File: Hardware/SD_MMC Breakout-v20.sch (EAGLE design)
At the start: 8 parts, among them U1 SD_CARD_SOCKET4UCON

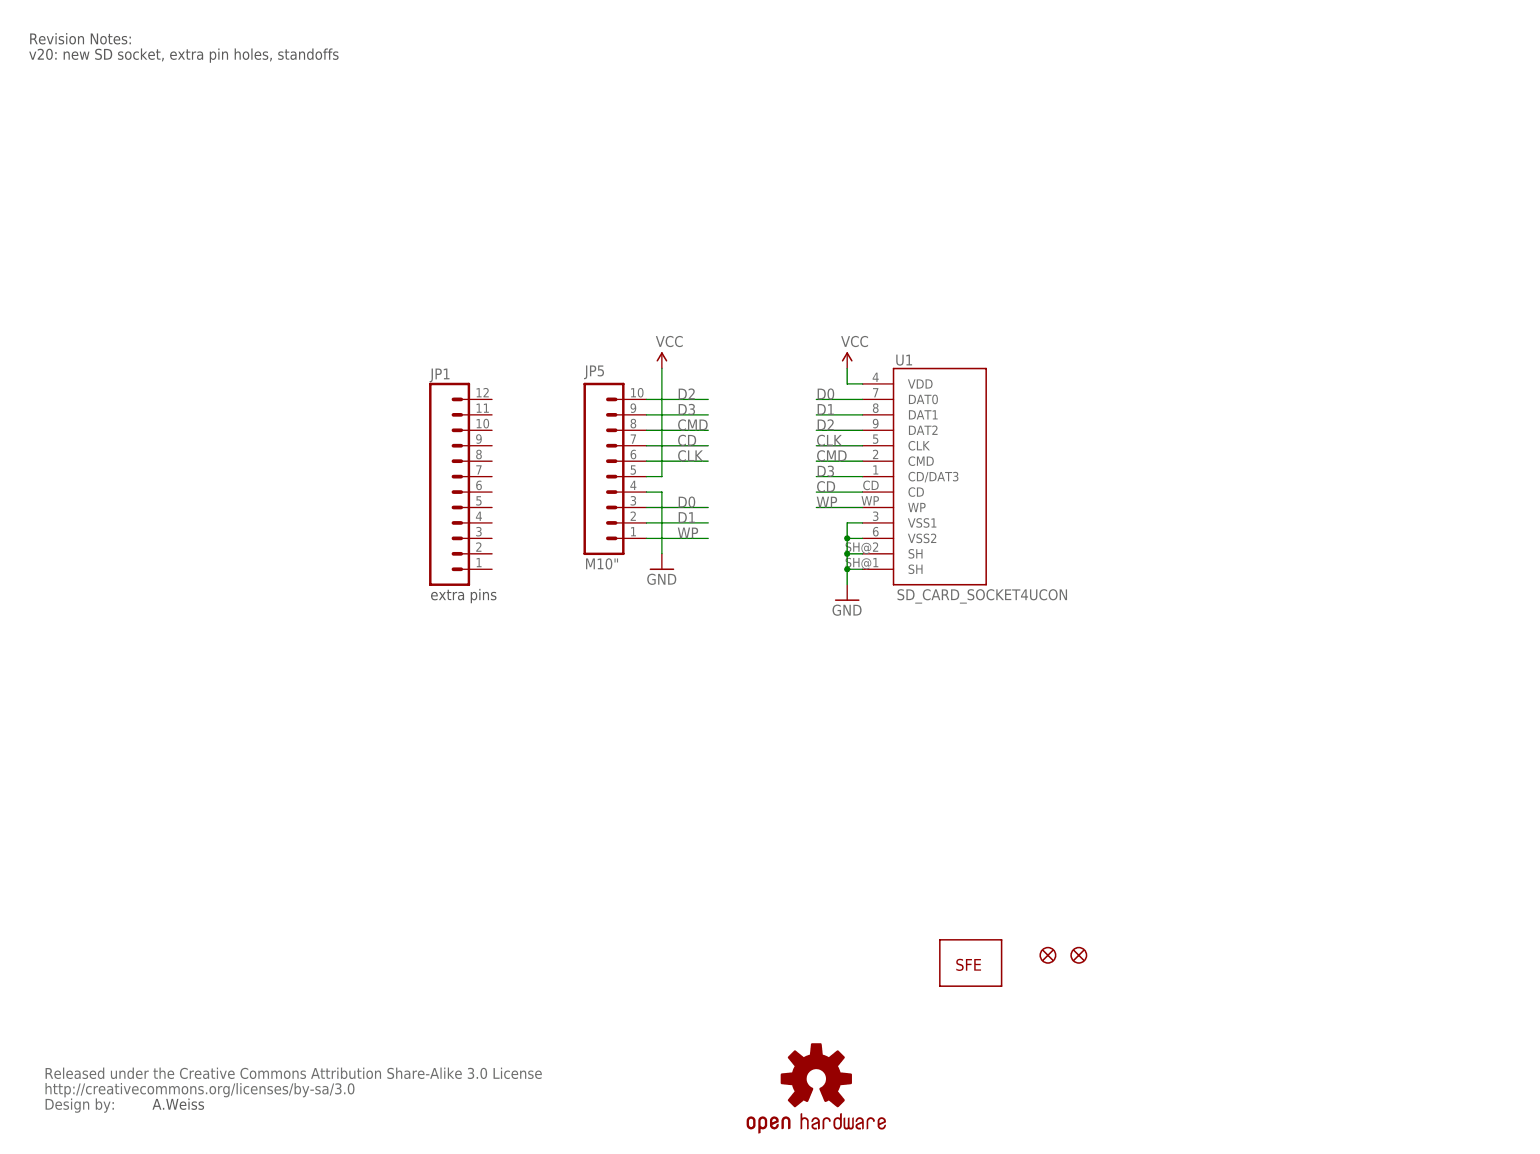
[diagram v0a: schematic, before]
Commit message: Added standoffs, sch work
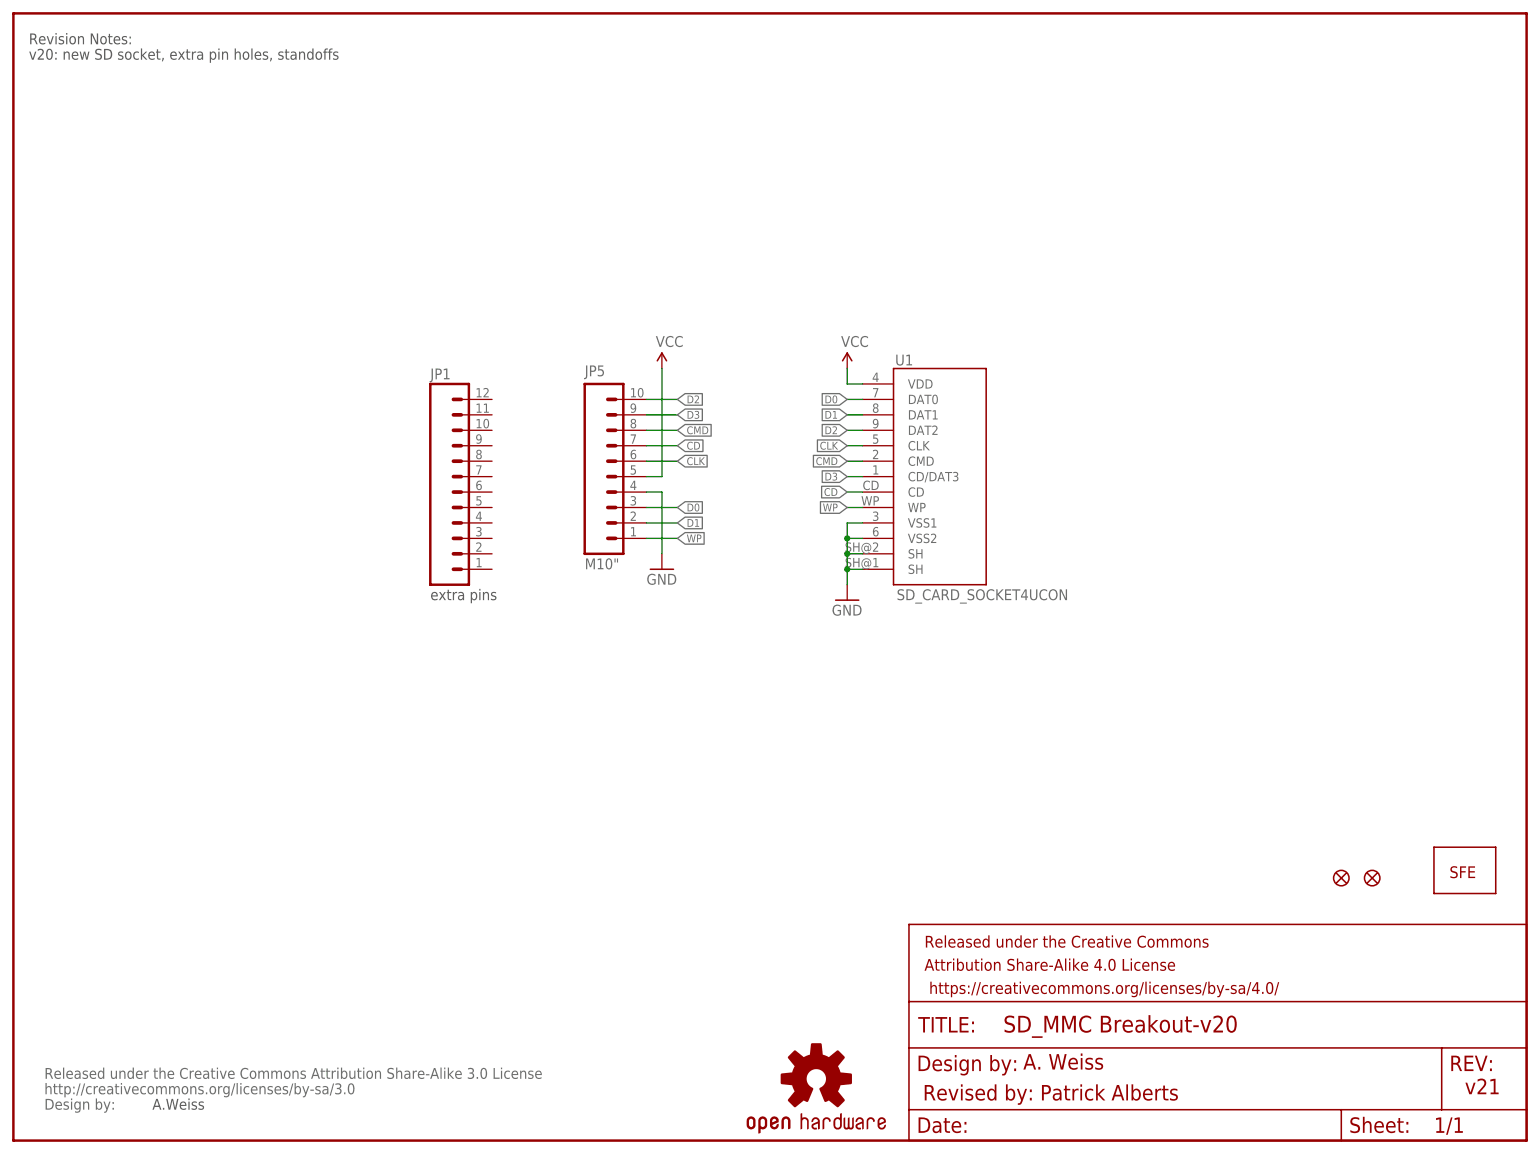
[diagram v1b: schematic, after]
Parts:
- added FRAME1: FRAME-LETTER, SparkFun-Aesthetics:FRAME-LETTER
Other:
- note added: "A. Weiss"
- note added: "Revised by: Patrick Alberts"
- note added: "v21"
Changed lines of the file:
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@@
 <?xml version="1.0" encoding="utf-8"?>
 <!DOCTYPE eagle SYSTEM "eagle.dtd">
-<eagle version="6.4">
+<eagle version="6.5.0">
 <drawing>
 <settings>
@@
 <layer number="106" name="bPlate" color="7" fill="1" visible="no" active="yes"/>
 <layer number="107" name="Crop" color="7" fill="1" visible="no" active="yes"/>
+<layer number="108" name="tplace-old" color="10" fill="1" visible="no" active="yes"/>
+<layer number="109" name="ref-old" color="11" fill="1" visible="no" active="yes"/>
 <layer number="116" name="Patch_BOT" color="9" fill="4" visible="yes" active="yes"/>
 <layer number="121" name="_tsilk" color="7" fill="1" visible="yes" active="yes"/>
@@
 <layer number="144" name="Drill_legend" color="7" fill="1" visible="no" active="yes"/>
 <layer number="151" name="HeatSink" color="7" fill="1" visible="yes" active="yes"/>
+<layer number="199" name="Contour" color="7" fill="1" visible="yes" active="yes"/>
 <layer number="200" name="200bmp" color="1" fill="10" visible="no" active="no"/>
 <layer number="201" name="201bmp" color="2" fill="1" visible="no" active="no"/>
@@
 </classes>
 <parts>
-<part name="FRAME1" library="SparkFun" deviceset="FRAME-LETTER" device=""/>
+<part name="FRAME1" library="SparkFun-Aesthetics" deviceset="FRAME-LETTER" device=""/>
 <part name="U$1" library="SparkFun" deviceset="LOGO-SFE" device="NEW"/>
 <part name="U1" library="SparkFun-Connectors" deviceset="SD_CARD_SOCKET" device="4UCON"/>
@@
 <text x="2.54" y="177.8" size="1.778" layer="97">v20: new SD socket, extra pin holes, standoffs</text>
 <text x="68.58" y="88.9" size="1.778" layer="97">extra pins</text>
+<text x="166.116" y="11.684" size="2.54" layer="94">A. Weiss</text>
+<text x="149.606" y="6.604" size="2.54" layer="94">Revised by: Patrick Alberts</text>
+<text x="238.76" y="7.62" size="2.54" layer="94">v21</text>
 </plain>
 <instances>
 <instance part="FRAME1" gate="G$1" x="0" y="0"/>
 <instance part="FRAME1" gate="G$2" x="147.32" y="0"/>
-<instance part="U$1" gate="G$1" x="154.94" y="27.94"/>
+<instance part="U$1" gate="G$1" x="236.22" y="43.18"/>
 <instance part="U1" gate="G$1" x="152.4" y="109.22" smashed="yes">
 <attribute name="NAME" x="145.034" y="127.508" size="1.778" layer="95"/>
@@
 <instance part="U$3" gate="G$1" x="132.08" y="10.16"/>
 <instance part="JP5" gate="G$1" x="93.98" y="116.84"/>
-<instance part="JP2" gate="G$1" x="170.18" y="30.48"/>
-<instance part="JP3" gate="G$1" x="175.26" y="30.48"/>
+<instance part="JP2" gate="G$1" x="218.44" y="43.18"/>
+<instance part="JP3" gate="G$1" x="223.52" y="43.18"/>
 </instances>
 <busses>
@@
 <segment>
 <pinref part="U1" gate="G$1" pin="CD"/>
-<wire x1="132.08" y1="106.68" x2="139.7" y2="106.68" width="0.1524" layer="91"/>
-<label x="132.08" y="106.68" size="1.778" layer="95"/>
-</segment>
-<segment>
-<wire x1="104.14" y1="114.3" x2="114.3" y2="114.3" width="0.1524" layer="91"/>
-<label x="109.22" y="114.3" size="1.778" layer="95"/>
+<wire x1="137.16" y1="106.68" x2="139.7" y2="106.68" width="0.1524" layer="91"/>
+<label x="137.16" y="106.68" size="1.27" layer="95" rot="R180" xref="yes"/>
+</segment>
+<segment>
+<wire x1="104.14" y1="114.3" x2="109.22" y2="114.3" width="0.1524" layer="91"/>
 <pinref part="JP5" gate="G$1" pin="7"/>
+<label x="109.22" y="114.3" size="1.27" layer="95" xref="yes"/>
 </segment>
 </net>
@@
 <segment>
 <pinref part="U1" gate="G$1" pin="CMD"/>
-<wire x1="132.08" y1="111.76" x2="139.7" y2="111.76" width="0.1524" layer="91"/>
-<label x="132.08" y="111.76" size="1.778" layer="95"/>
-</segment>
-<segment>
-<wire x1="104.14" y1="116.84" x2="114.3" y2="116.84" width="0.1524" layer="91"/>
-<label x="109.22" y="116.84" size="1.778" layer="95"/>
+<wire x1="137.16" y1="111.76" x2="139.7" y2="111.76" width="0.1524" layer="91"/>
+<label x="137.16" y="111.76" size="1.27" layer="95" rot="R180" xref="yes"/>
+</segment>
+<segment>
+<wire x1="104.14" y1="116.84" x2="109.22" y2="116.84" width="0.1524" layer="91"/>
 <pinref part="JP5" gate="G$1" pin="8"/>
+<label x="109.22" y="116.84" size="1.27" layer="95" xref="yes"/>
 </segment>
 </net>
@@
 <segment>
 <pinref part="U1" gate="G$1" pin="CLK"/>
-<wire x1="132.08" y1="114.3" x2="139.7" y2="114.3" width="0.1524" layer="91"/>
-<label x="132.08" y="114.3" size="1.778" layer="95"/>
-</segment>
-<segment>
-<wire x1="104.14" y1="111.76" x2="114.3" y2="111.76" width="0.1524" layer="91"/>
-<label x="109.22" y="111.76" size="1.778" layer="95"/>
+<wire x1="137.16" y1="114.3" x2="139.7" y2="114.3" width="0.1524" layer="91"/>
+<label x="137.16" y="114.3" size="1.27" layer="95" rot="R180" xref="yes"/>
+</segment>
+<segment>
+<wire x1="104.14" y1="111.76" x2="109.22" y2="111.76" width="0.1524" layer="91"/>
 <pinref part="JP5" gate="G$1" pin="6"/>
+<label x="109.22" y="111.76" size="1.27" layer="95" xref="yes"/>
 </segment>
 </net>
@@
 <segment>
 <pinref part="U1" gate="G$1" pin="DAT1"/>
-<wire x1="132.08" y1="119.38" x2="139.7" y2="119.38" width="0.1524" layer="91"/>
-<label x="132.08" y="119.38" size="1.778" layer="95"/>
-</segment>
-<segment>
-<wire x1="104.14" y1="101.6" x2="114.3" y2="101.6" width="0.1524" layer="91"/>
-<label x="109.22" y="101.6" size="1.778" layer="95"/>
+<wire x1="137.16" y1="119.38" x2="139.7" y2="119.38" width="0.1524" layer="91"/>
+<label x="137.16" y="119.38" size="1.27" layer="95" rot="R180" xref="yes"/>
+</segment>
+<segment>
+<wire x1="104.14" y1="101.6" x2="109.22" y2="101.6" width="0.1524" layer="91"/>
 <pinref part="JP5" gate="G$1" pin="2"/>
+<label x="109.22" y="101.6" size="1.27" layer="95" xref="yes"/>
 </segment>
 </net>
@@
 <segment>
 <pinref part="U1" gate="G$1" pin="DAT0"/>
-<wire x1="132.08" y1="121.92" x2="139.7" y2="121.92" width="0.1524" layer="91"/>
-<label x="132.08" y="121.92" size="1.778" layer="95"/>
-</segment>
-<segment>
-<wire x1="104.14" y1="104.14" x2="114.3" y2="104.14" width="0.1524" layer="91"/>
-<label x="109.22" y="104.14" size="1.778" layer="95"/>
+<wire x1="137.16" y1="121.92" x2="139.7" y2="121.92" width="0.1524" layer="91"/>
+<label x="137.16" y="121.92" size="1.27" layer="95" rot="R180" xref="yes"/>
+</segment>
+<segment>
+<wire x1="104.14" y1="104.14" x2="109.22" y2="104.14" width="0.1524" layer="91"/>
 <pinref part="JP5" gate="G$1" pin="3"/>
+<label x="109.22" y="104.14" size="1.27" layer="95" xref="yes"/>
 </segment>
 </net>
@@
 <segment>
 <pinref part="U1" gate="G$1" pin="WP"/>
-<wire x1="139.7" y1="104.14" x2="132.08" y2="104.14" width="0.1524" layer="91"/>
-<label x="132.08" y="104.14" size="1.778" layer="95"/>
+<wire x1="139.7" y1="104.14" x2="137.16" y2="104.14" width="0.1524" layer="91"/>
+<label x="137.16" y="104.14" size="1.27" layer="95" rot="R180" xref="yes"/>
 </segment>
 <segment>
 <pinref part="JP5" gate="G$1" pin="1"/>
-<wire x1="104.14" y1="99.06" x2="114.3" y2="99.06" width="0.1524" layer="91"/>
-<label x="109.22" y="99.06" size="1.778" layer="95"/>
+<wire x1="104.14" y1="99.06" x2="109.22" y2="99.06" width="0.1524" layer="91"/>
+<label x="109.22" y="99.06" size="1.27" layer="95" xref="yes"/>
 </segment>
 </net>
@@
 <segment>
 <pinref part="U1" gate="G$1" pin="DAT2"/>
-<wire x1="132.08" y1="116.84" x2="139.7" y2="116.84" width="0.1524" layer="91"/>
-<label x="132.08" y="116.84" size="1.778" layer="95"/>
-</segment>
-<segment>
-<wire x1="104.14" y1="121.92" x2="114.3" y2="121.92" width="0.1524" layer="91"/>
-<label x="109.22" y="121.92" size="1.778" layer="95"/>
+<wire x1="137.16" y1="116.84" x2="139.7" y2="116.84" width="0.1524" layer="91"/>
+<label x="137.16" y="116.84" size="1.27" layer="95" rot="R180" xref="yes"/>
+</segment>
+<segment>
+<wire x1="104.14" y1="121.92" x2="109.22" y2="121.92" width="0.1524" layer="91"/>
 <pinref part="JP5" gate="G$1" pin="10"/>
+<label x="109.22" y="121.92" size="1.27" layer="95" xref="yes"/>
 </segment>
 </net>
@@
 <segment>
 <pinref part="U1" gate="G$1" pin="CD/DAT3"/>
-<wire x1="132.08" y1="109.22" x2="139.7" y2="109.22" width="0.1524" layer="91"/>
-<label x="132.08" y="109.22" size="1.778" layer="95"/>
-</segment>
-<segment>
-<wire x1="104.14" y1="119.38" x2="114.3" y2="119.38" width="0.1524" layer="91"/>
-<label x="109.22" y="119.38" size="1.778" layer="95"/>
+<wire x1="137.16" y1="109.22" x2="139.7" y2="109.22" width="0.1524" layer="91"/>
+<label x="137.16" y="109.22" size="1.27" layer="95" rot="R180" xref="yes"/>
+</segment>
+<segment>
+<wire x1="104.14" y1="119.38" x2="109.22" y2="119.38" width="0.1524" layer="91"/>
 <pinref part="JP5" gate="G$1" pin="9"/>
-</segment>
-</net>
+<label x="109.22" y="119.38" size="1.27" layer="95" xref="yes"/>
+</segment>
+</net>
